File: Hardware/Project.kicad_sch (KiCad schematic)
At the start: 25 parts, among them IC1 ESP32-S3-WROOM-1-N8, J1 USB_C_2.0, SW1 B3U-1000P, SW2 B3U-1000P, U2 TLV1117LV33DCYR

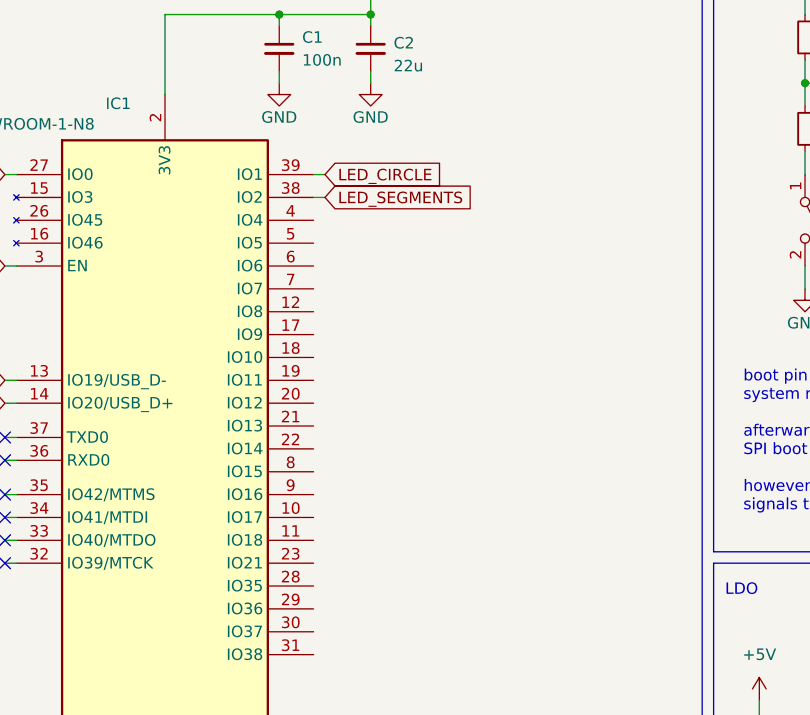
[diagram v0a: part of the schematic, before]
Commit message: Finished layout
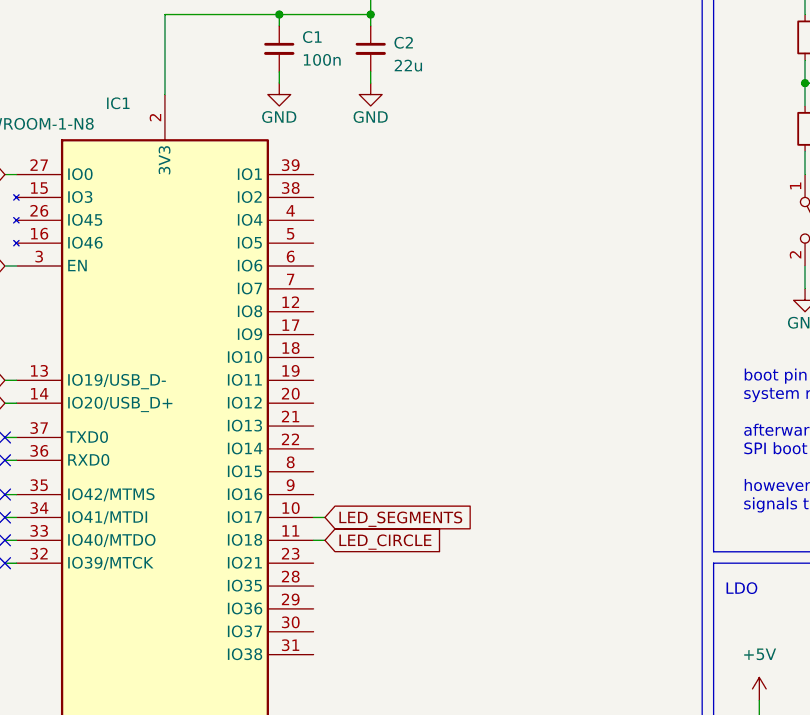
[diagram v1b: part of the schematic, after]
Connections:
- net LED_CIRCLE: now also IC1.11 (IO18); no longer IC1.39 (IO1)
- net LED_SEGMENTS: now also IC1.10 (IO17); no longer IC1.38 (IO2)
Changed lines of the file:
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@@
 	(wire
 		(pts
-			(xy 91.44 49.53) (xy 90.17 49.53)
+			(xy 91.44 87.63) (xy 90.17 87.63)
 		)
 		(stroke
@@
 	(wire
 		(pts
-			(xy 91.44 52.07) (xy 90.17 52.07)
+			(xy 91.44 90.17) (xy 90.17 90.17)
 		)
 		(stroke
@@
 	(global_label "LED_SEGMENTS"
 		(shape input)
-		(at 91.44 52.07 0)
+		(at 91.44 87.63 0)
 		(fields_autoplaced yes)
 		(effects
@@
 		)
 		(property "Intersheetrefs" "${INTERSHEET_REFS}"
-			(at 108.5764 52.07 0)
+			(at 108.5764 87.63 0)
 			(effects
 				(font
@@
 	(global_label "LED_CIRCLE"
 		(shape input)
-		(at 91.44 49.53 0)
+		(at 91.44 90.17 0)
 		(fields_autoplaced yes)
 		(effects
@@
 		)
 		(property "Intersheetrefs" "${INTERSHEET_REFS}"
-			(at 105.4318 49.53 0)
+			(at 105.4318 90.17 0)
 			(effects
 				(font
